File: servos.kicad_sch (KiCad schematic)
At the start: 19 parts, among them J10 Conn_01x03, J11 Conn_01x03, J6 Conn_01x03, J7 Conn_01x03, J8 Conn_01x03, J9 Conn_01x03, U10 INA745A, U11 INA745A, U12 INA745A, U13 INA745A, U6 INA745A, U9 INA745A

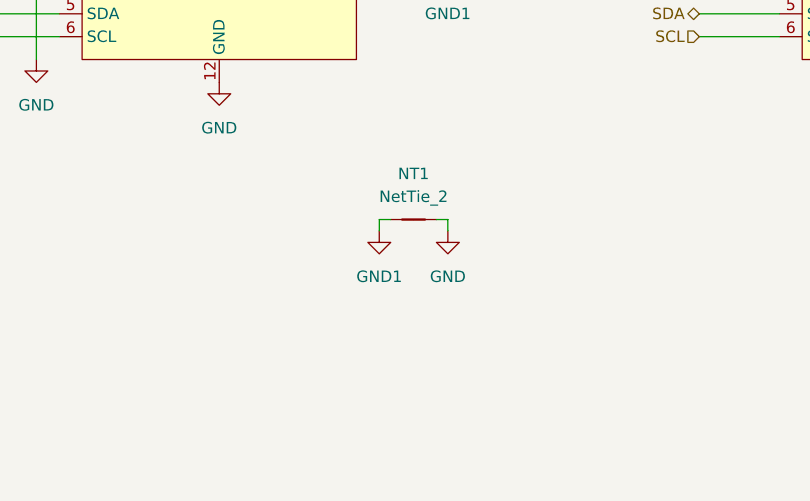
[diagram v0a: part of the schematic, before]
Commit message: add some TVS diodes
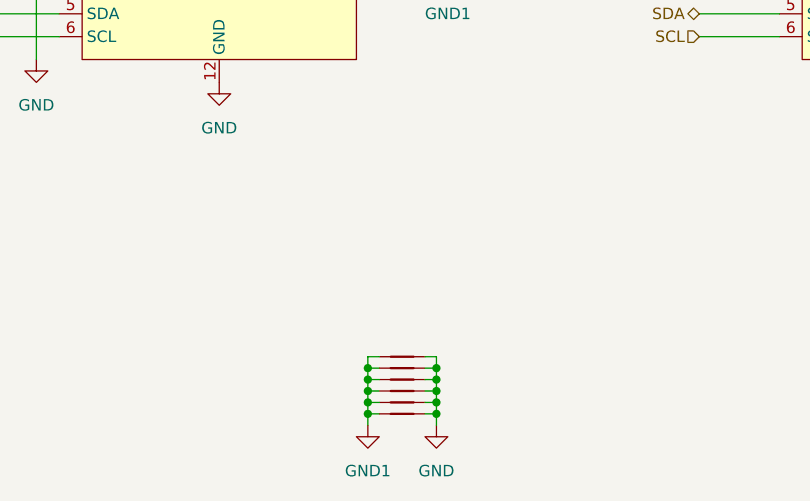
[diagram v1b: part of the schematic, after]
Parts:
- added NT2, NT3, NT4, NT5, NT6: NetTie_2, NetTie:NetTie-2_SMD_Pad2.0mm, symbol Device:NetTie_2
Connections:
- net GND: now also NT2.2, NT3.2, NT4.2, NT5.2, NT6.2
- net GND1: now also NT2.1, NT3.1, NT4.1, NT5.1, NT6.1
